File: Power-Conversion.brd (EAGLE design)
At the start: 185.4 x 81.3 mm, 70 parts, among them J1 AVR_SPI_PRG_6PTH, U1 ATMEGA328P_TQFP, U2 LM1085IS-3.3

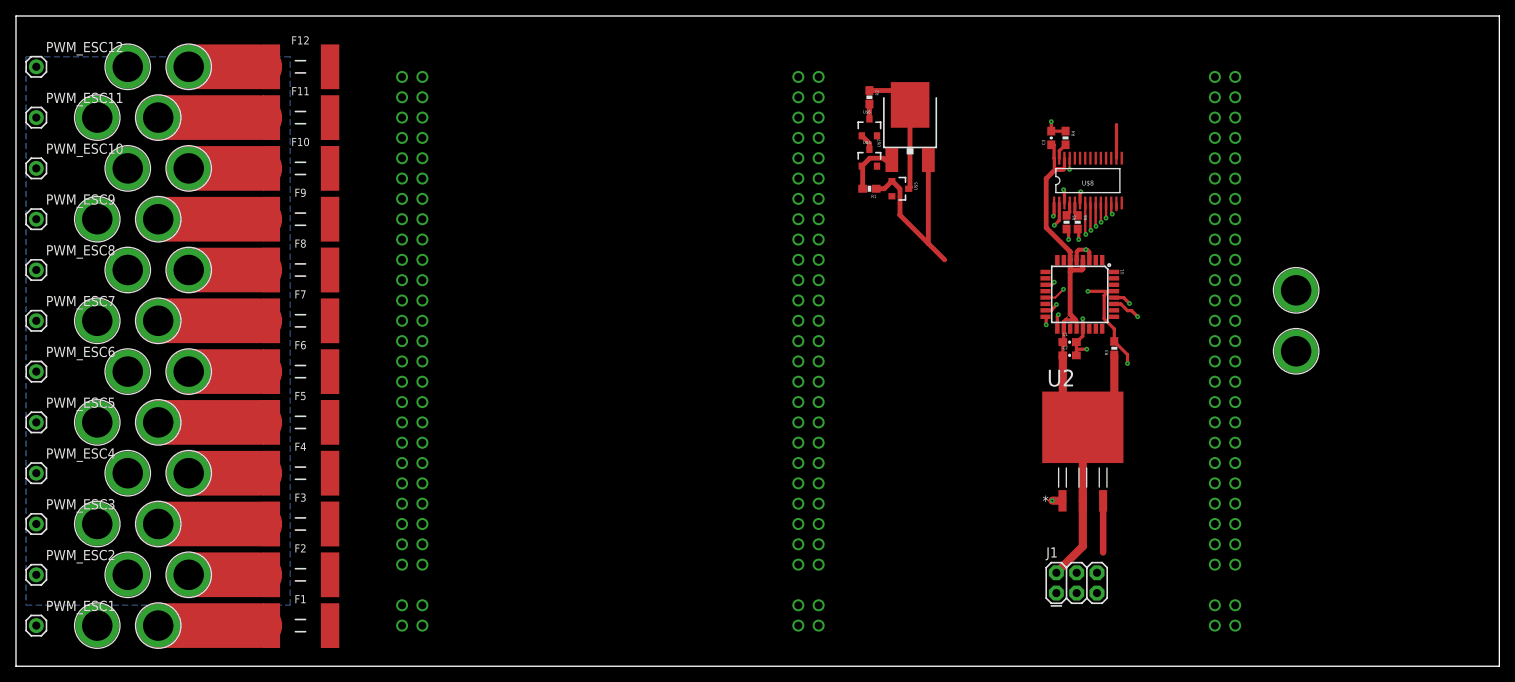
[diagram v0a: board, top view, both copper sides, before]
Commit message: After 8 hours of continuous work, I am 90% done with the power distribution board
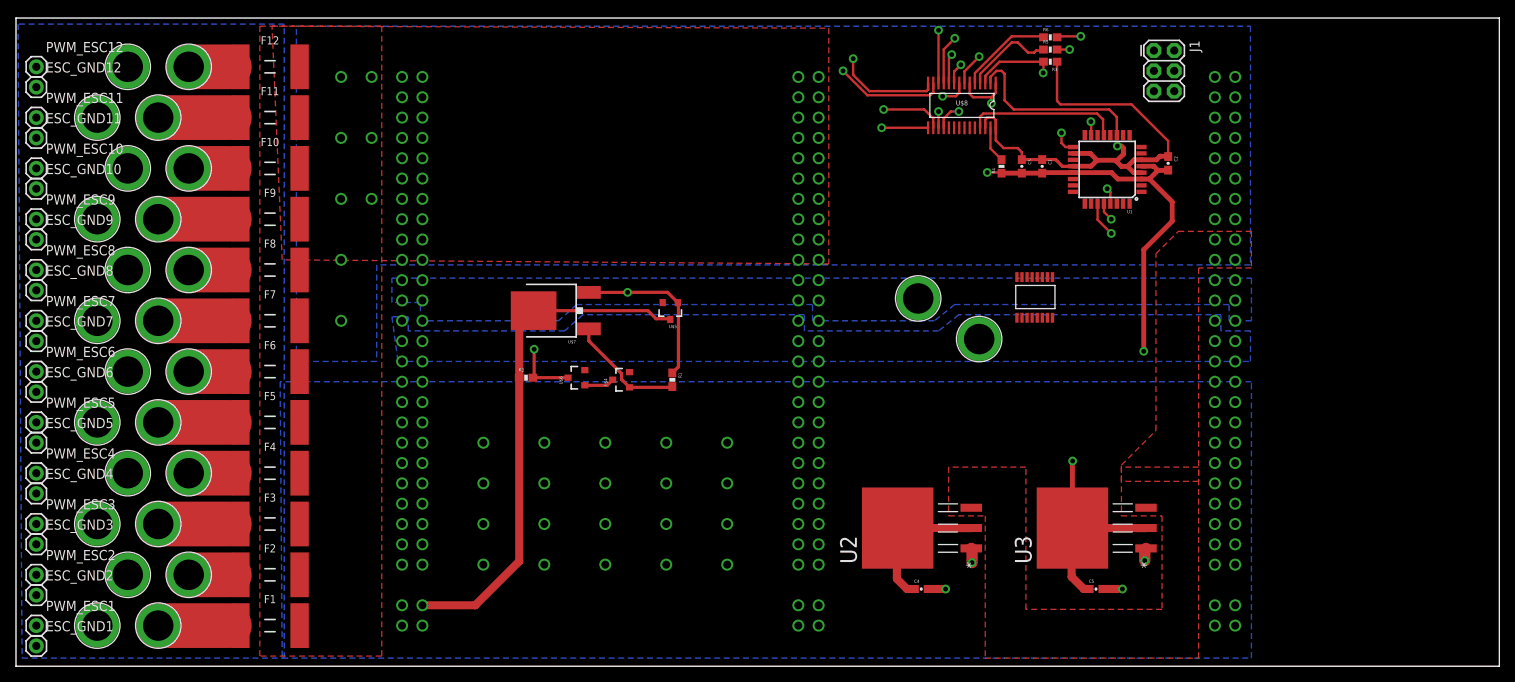
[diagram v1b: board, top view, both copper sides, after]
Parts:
- added C4, C5: 1uF, SparkFun-Capacitors:0603-CAP
- added ESC_GND1, ESC_GND10, ESC_GND11, ESC_GND12, ESC_GND2, ESC_GND3, ESC_GND4, ESC_GND5, ESC_GND6, ESC_GND7, ESC_GND8, ESC_GND9: (no value), SparkFun-Connectors:1X01
- added U$9: FT230XS, USB-UART:SSOP-16
- added U3: LM1085IS-3.3, PowerComponents:TO254P1435X457-3N
- moved J1 68.9 mm to (142.2, 77.0), turned to 270 degrees
- moved R2 55.4 mm to (63.8, 36.1), turned to 0 degrees
- moved U$7 51.5 mm to (66.3, 44.5), turned to 90 degrees
- moved U$6 48.1 mm to (70.1, 36.1), turned to 90 degrees
- moved V-_CONN 47.3 mm to (112.8, 46.0)
- moved U$4 41.6 mm to (75.7, 35.8), turned to 90 degrees
- moved V+_CONN 39.7 mm to (120.4, 40.9)
- moved R3 36.7 mm to (129.3, 75.6), turned to 180 degrees
- moved R1 34.3 mm to (82.0, 35.8), turned to 270 degrees
- moved U$5 32.5 mm to (81.8, 44.5), turned to 180 degrees
- moved C2 27.0 mm to (144.0, 62.9), turned to 270 degrees
- moved U2 26.1 mm to (110.4, 17.3), turned to 90 degrees
- moved R6 23.4 mm to (129.3, 78.6), turned to 0 degrees
- moved C1 22.2 mm to (128.3, 62.5), turned to 270 degrees
- moved R5 21.7 mm to (129.3, 77.1), turned to 0 degrees
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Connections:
- new net +5_SERVO: C4.1, U2.2, U2.4
- net +5V: now also C5.1, U3.2, U3.4; no longer U2.2, U2.4
- net GND: now also C4.2, C5.2, ESC_GND1.1, ESC_GND10.1, ESC_GND11.1, ESC_GND12.1, ESC_GND2.1, ESC_GND3.1, ESC_GND4.1, ESC_GND5.1, ESC_GND6.1, ESC_GND7.1, ESC_GND8.1, ESC_GND9.1, U$9.P$13, U$9.P$5, U3.1
- net VCC: now also U3.3
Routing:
- net SDA: track 3.61 -> 174.0 mm
- net SCL: track 5.15 -> 174.4 mm
- net N$15: track 39.3 -> 203.4 mm
- net N$16: track 32.6 -> 186.1 mm
- net ONOFF: track 16.4 -> 167.7 mm
- net N$21: track 0.90 -> 151.9 mm, vias 0 -> 1
- net N$18: track 21.9 -> 172.1 mm
- net N$19: track 18.0 -> 168.2 mm
- net N$17: track 28.4 -> 178.4 mm
- net N$20: track 11.4 -> 160.8 mm
- net N$22: track 0.00 -> 144.8 mm, vias 0 -> 1
- net N$23: track 0.00 -> 142.7 mm, vias 0 -> 1
- net N$2: track 0.00 -> 135.3 mm, vias 0 -> 1
- net N$4: track 0.00 -> 134.5 mm, vias 0 -> 1
- net N$24: track 4.20 -> 137.5 mm, vias 0 -> 1
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- added copper zone on layer 15, net GND
- added copper zone on layer 2, net GND
- added copper zone on layer 16, net V+
- added copper zone on layer 16, net V-
- added copper zone on layer 1, net VCC
- added copper zone on layer 16, net VCC
- removed copper zone on layer 1, net +5V
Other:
- board size 185.4 x 81.3 mm -> 185.4 x 81 mm
